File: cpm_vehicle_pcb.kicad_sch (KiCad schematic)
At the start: 71 parts, among them IC1 ATMEGAAU, IC2 RPI-ZERO, J1 Conn_02x03_Counter_Clockwise, J2 Conn_02x03_Counter_Clockwise, J3 Conn_01x05, J5 USB_B_Mini, J6 Conn_01x03_Socket, P1 NCP1117, Q11 BSS123, Q12 BSS123, Q13 BSS123, Q14 BSS123, Q3 DMG9926UDM, SW1 SW_DIP_x02, SW2 SW_SPDT_312, U3 TXB0104PWR, U4 MT3608, U7 CH340G, U8 R5460N

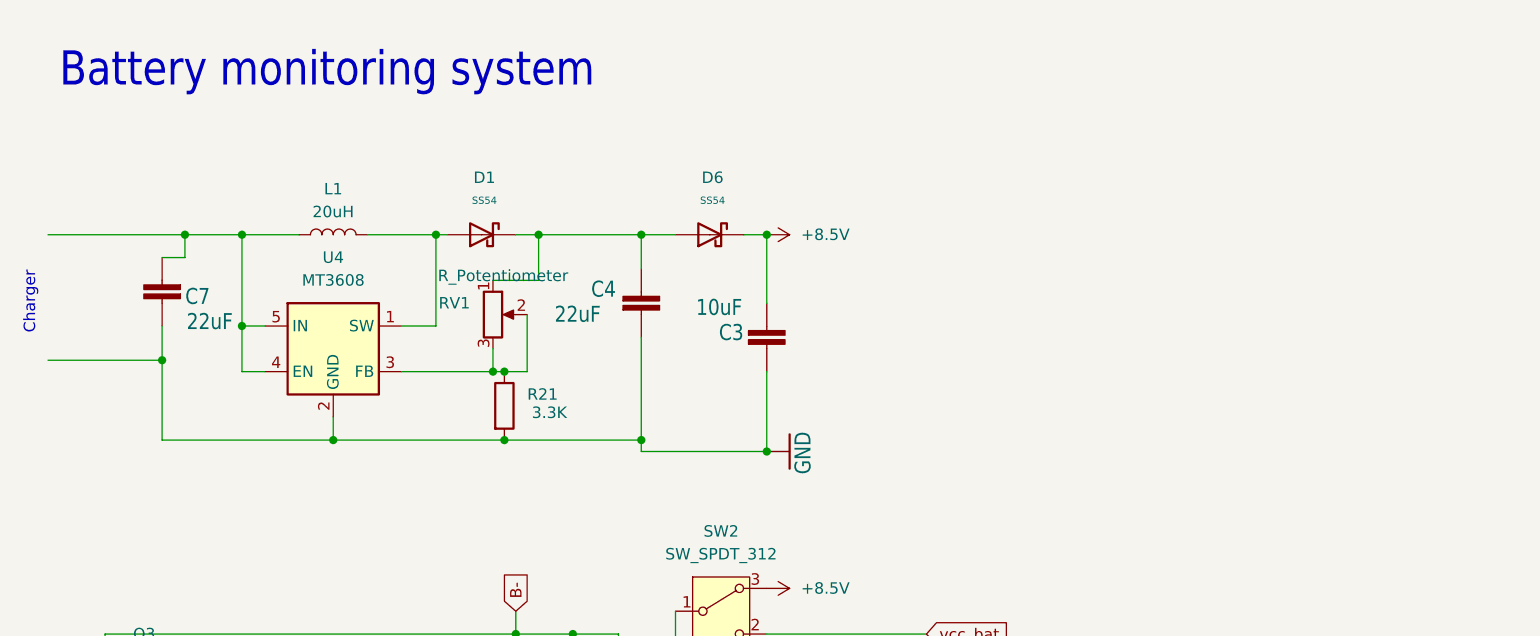
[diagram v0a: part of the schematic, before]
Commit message: update
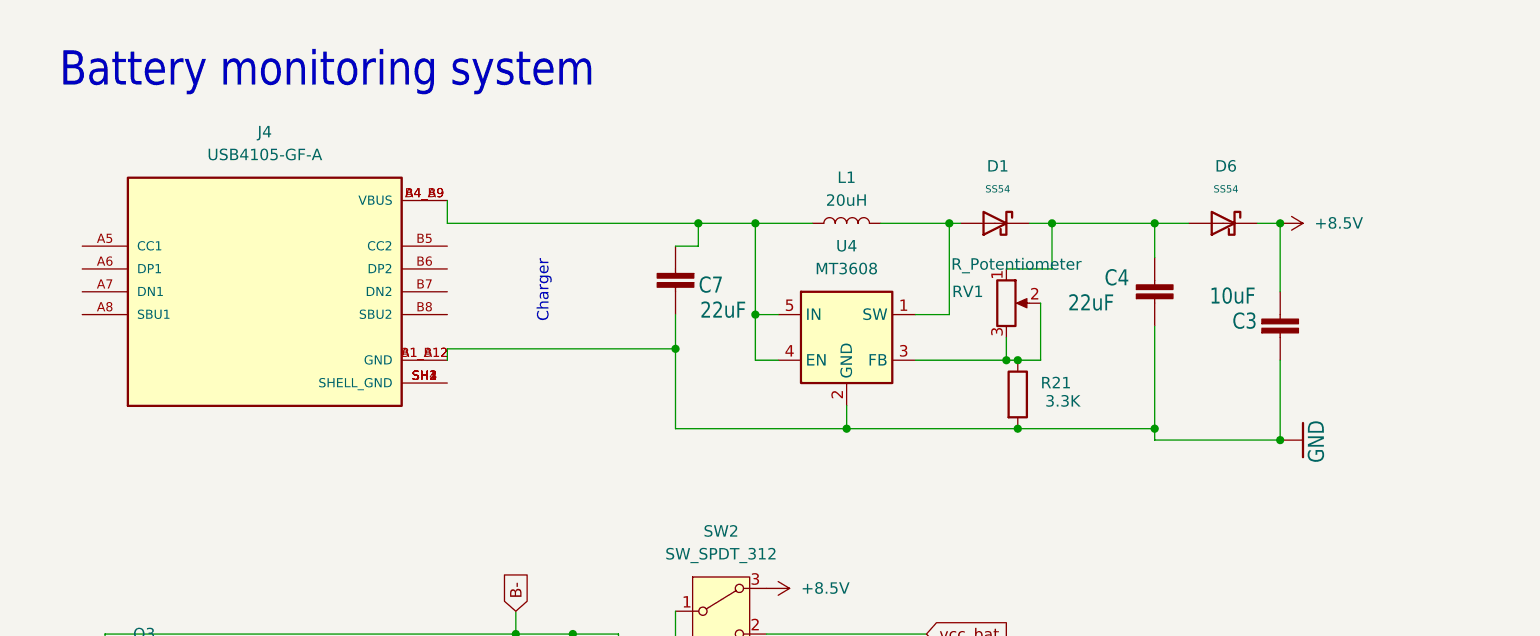
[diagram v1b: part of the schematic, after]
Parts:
- added J4: USB4105-GF-A, footprints_vehicle_pcb:GCT_USB4105-GF-A, symbol USBC:USB4105-GF-A
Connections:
- net GND: now also J4.A1_B12 (GND), J4.B1_A12 (GND)
- net at C7.2, L1.1, U4.4 (EN)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: now also J4.A4_B9 (VBUS), J4.B4_A9 (VBUS)
- new net: J4.SH1 (SHELL_GND), J4.SH2 (SHELL_GND), J4.SH3 (SHELL_GND), J4.SH4 (SHELL_GND)
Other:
- moved on the sheet: C3, C4, C7, D1, D6, L1, R21, RV1, U4
